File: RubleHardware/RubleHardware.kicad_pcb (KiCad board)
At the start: 4 copper layers, 52 x 50 mm, 49 parts, among them IC1 LTC3780EUH#PBF, J1_IN1 Conn_01x08_Male, J2_OUT1 Conn_01x08_Male

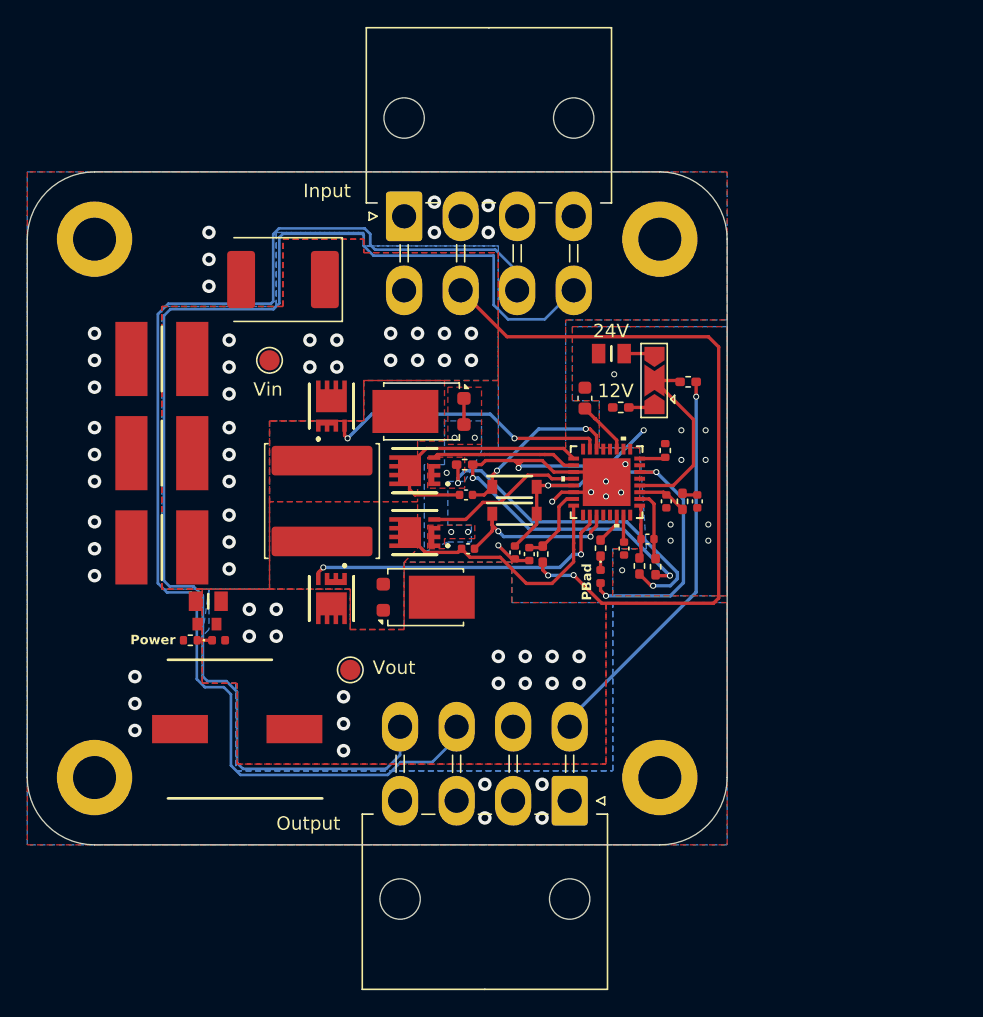
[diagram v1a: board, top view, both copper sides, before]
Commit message: trying something out
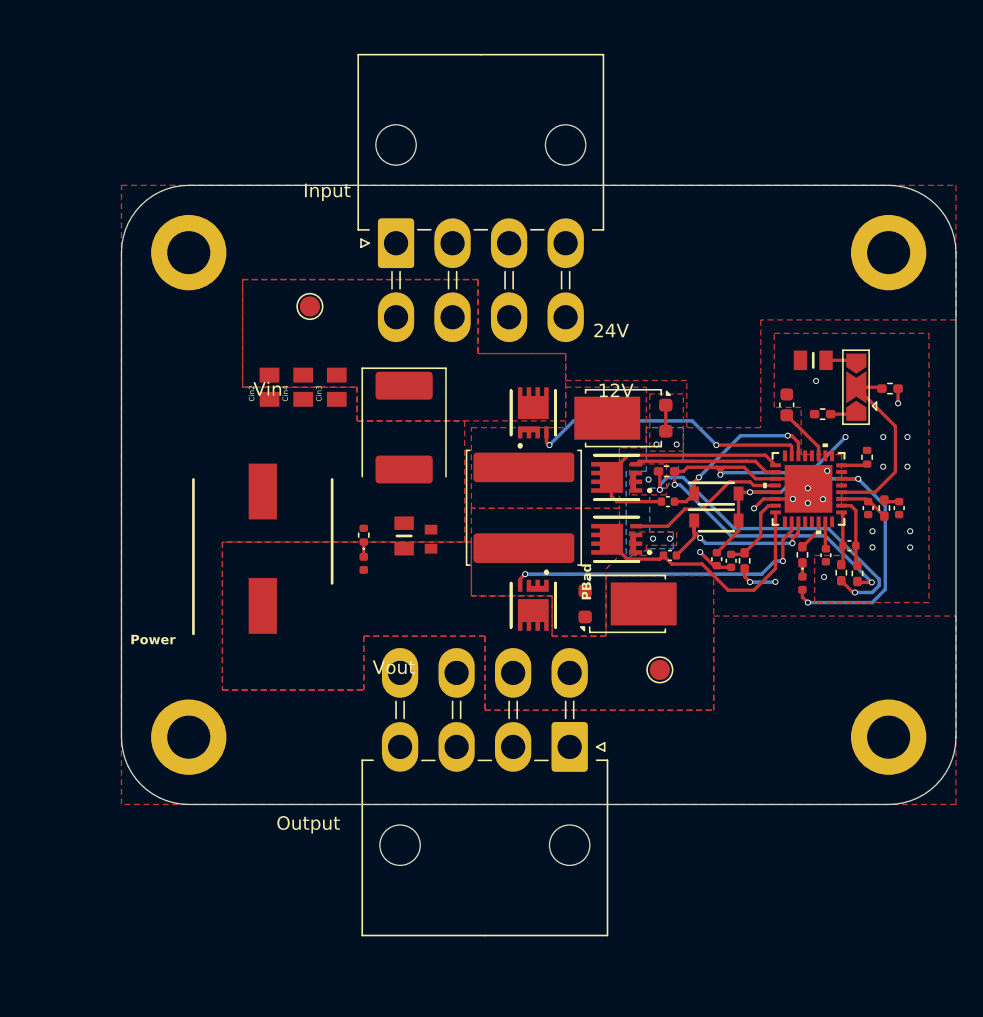
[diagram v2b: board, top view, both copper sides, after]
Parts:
- Cin2, Cin3, Cin4: footprint iclr:CAPC6050X550N -> iclr:CAPC2012X145N
- moved TP1 23.0 mm to (173.0, 102.0)
- moved Cout1 17.8 mm to (156.0, 92.3), turned to 90 degrees
- moved Cin3 17.6 mm to (149.0, 81.0), turned to 90 degrees
- moved H4 17.3 mm to (190.0, 107.0)
- moved H3 17.0 mm to (190.0, 71.0)
- moved Cout3 15.3 mm to (154.0, 92.0), turned to 90 degrees
- moved R3 15.1 mm to (151.0, 92.0), turned to 90 degrees
- moved A1 15.0 mm to (163.6, 82.9)
- moved B1 15.0 mm to (169.8, 87.7)
- moved C1 15.0 mm to (190.8, 90.0)
- moved C2 15.0 mm to (188.5, 90.0)
- moved C3 15.0 mm to (169.8, 92.3)
- moved C4 15.0 mm to (182.4, 82.3)
- moved CSENS1 15.0 mm to (187.1, 92.8)
- moved Ca1 15.0 mm to (173.7, 93.5)
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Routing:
- net /CAN+: track 95.4 -> 0.00 mm
- net /CAN-: track 92.1 -> 0.00 mm
- net /ICVIN: track 54.5 -> 3.09 mm, vias 23 -> 2
- net /ICVOUT: track 29.5 -> 1.10 mm, vias 16 -> 1
- net GND: vias 44 -> 21
- removed copper zone on In2.Cu, net +3V3
- removed copper zone on B.Cu, net /ICVIN
- removed copper zone on B.Cu, net /ICVOUT
- removed copper zone on B.Cu, net GND
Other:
- board size 52 x 50 mm -> 62 x 46 mm
